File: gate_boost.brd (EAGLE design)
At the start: 74.9 x 45.3 mm, 57 parts, among them IC1 LM324D, IC2 SP34063A_BOOST_REG

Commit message: prior change to charge pump
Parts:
- C1: value (none) -> 1500pf
- R19: value (none) -> 68k
- R20: value (none) -> 180
- R21: value (none) -> 0.22
- R23: value (none) -> 3k3
- R24: value (none) -> 6k2

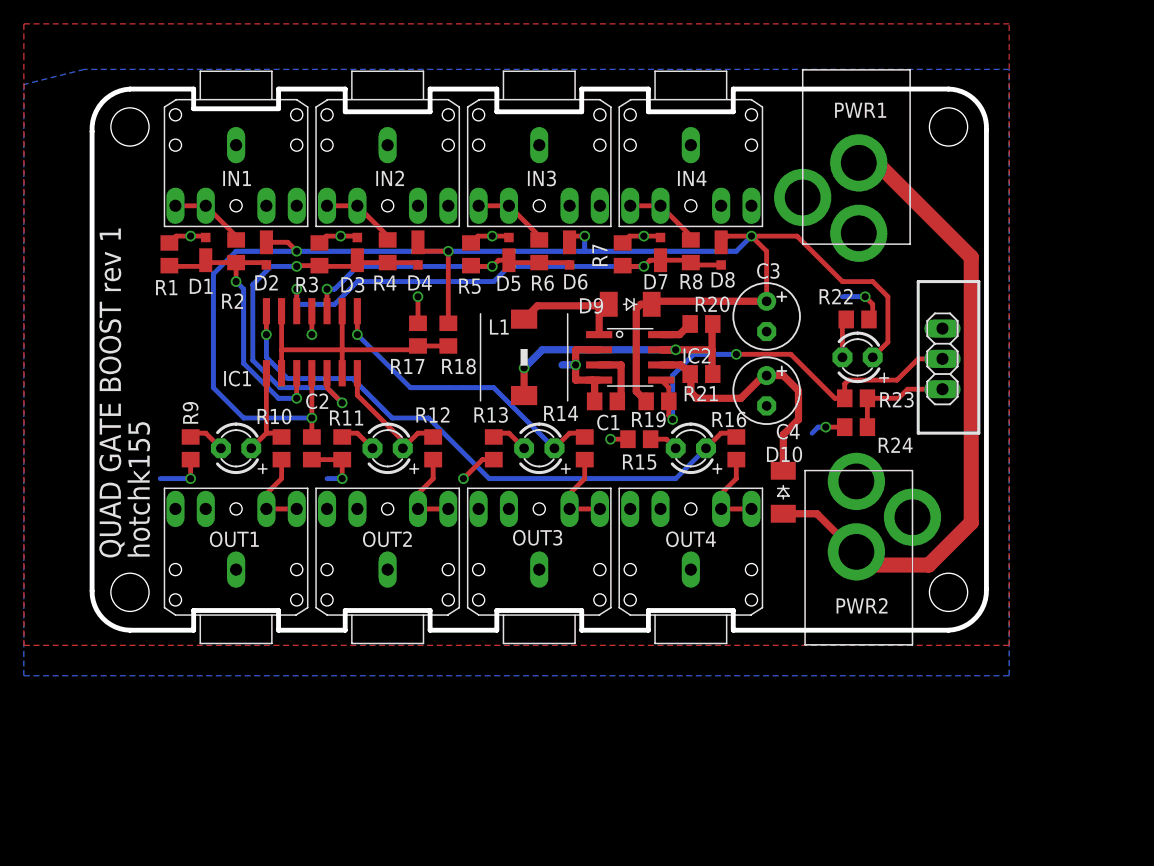
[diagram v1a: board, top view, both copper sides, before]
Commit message: charge pump
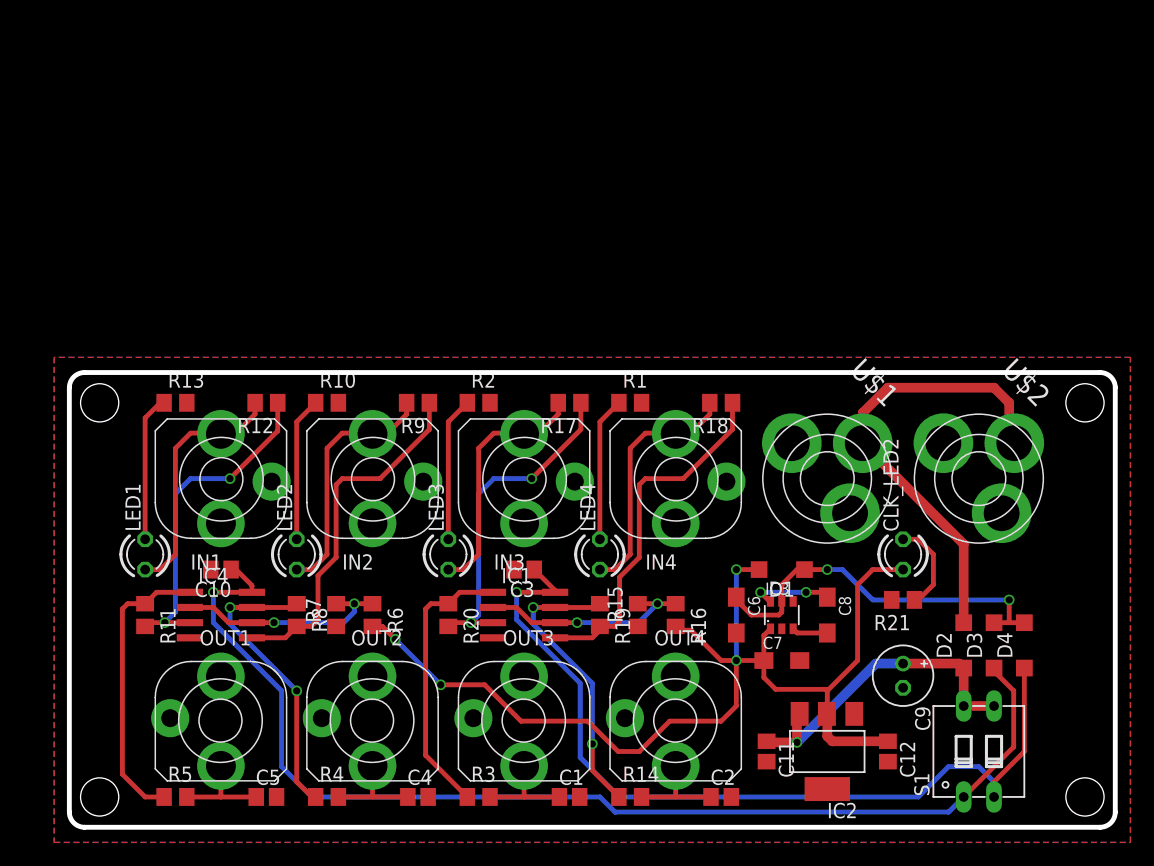
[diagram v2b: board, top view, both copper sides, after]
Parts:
- removed D10, D9: CGRM4001-G, diode:SOD-123_MINI-SMA
- removed D5, D6, D7, D8: PD3S160, diode:POWERDI323
- removed JP1: (no value), pinhead:1X03
- removed L1: (no value), wuerth-elektronik:WE-PD_S/M
- removed LED5: (no value), adafruit:LED3MM
- removed PWR1, PWR2: 2.1MMJACKTHM, adafruit:PJ-102A
- removed R22: (no value), rcl:R0805
- removed R23: 3k3, rcl:R0805
- removed R24: 6k2, rcl:R0805
- added C10, C11, C12, C5: (no value), resistor:C0805
- added C6: (no value), rcl:SMC_A
- added C7, C8: 10u, rcl:SMC_A
- added C9: (no value), rcl:E2-5
- added CLK_LED2: (no value), led:LED3MM
- added IC3: LM27675M5_CHARGEPUMP, jason_eagle6:SOT23-6
- added IC4: LM358D, linear:SO08
- added S1: (no value), switch-dil:DIP02YL
- added U$1, U$2: PWR_SOCKET_2_1MM, jason_eagle6:PWR_SOCKET_2_1MM
- C1: value 1500pf -> (none); device rcl:C0805 -> resistor:C0805
- C2: device rcl:C0805 -> resistor:C0805
- C3, C4: device rcl:E2,5-6 -> resistor:C0805
- D1, D2, D3, D4: value PD3S160 -> MBR0520LT; device diode:POWERDI323 -> diode:SOD123
- IC1: value LM324D -> LM358D; device linear:SO14 -> linear:SO08
- IC2: value SP34063A_BOOST_REG -> REG1117; device jason_eagle6:SOIC8 -> burr-brown:SOT223
- IN1, IN2, IN3, IN4, OUT1, OUT2, OUT3, OUT4: value TRUCONNECTJACK -> VERTICAL_3_5MM_SOCKET; device jason_eagle6:TRUCONNECTJACK -> jason_eagle6:VERTICAL_3_5MM_SOCKET
- LED1, LED2, LED3, LED4: device adafruit:LED3MM -> led:LED3MM
- R1, R10, R13, R2: value (none) -> 1K
- R12, R16, R17, R18, R6, R9: value (none) -> 100k
- R19: value 68k -> (none)
- R20: value 180 -> (none)
- R21: value 0.22 -> 1K
- moved D2 67.1 mm to (72.4, 27.9), turned to 90 degrees
- moved D3 62.7 mm to (74.9, 27.9)
- moved D4 60.6 mm to (77.5, 27.9), turned to 90 degrees
- moved D1 55.1 mm to (57.1, 34.3), turned to 180 degrees
- moved R5 51.8 mm to (6.35, 15.2), turned to 0 degrees
- moved R3 47.4 mm to (31.8, 15.2), turned to 0 degrees
- moved R4 46.0 mm to (19.1, 15.2), turned to 0 degrees
- moved C2 45.0 mm to (52.1, 15.2), turned to 0 degrees
- moved R8 44.9 mm to (16.5, 30.5)
- moved C4 44.9 mm to (26.7, 15.2), turned to 0 degrees
- moved R1 40.6 mm to (44.5, 48.3), turned to 0 degrees
- moved R7 38.6 mm to (19.8, 30.5), turned to 90 degrees
- moved IC2 36.9 mm to (61.0, 19.1), turned to 180 degrees
- moved R6 33.5 mm to (22.9, 30.5)
- moved C1 33.3 mm to (39.4, 15.2), turned to 0 degrees
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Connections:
- removed net N$18: IC1.8, LED3.A, R14.1
- removed net N$22: IC2.8, R20.1
- removed net N$24: C4.+, D10.C, IC2.6, R21.1
- removed net N$25: D10.A, PWR1.RING, PWR2.RING
- removed net N$27: LED1.K, R9.2
- removed net N$30: LED2.K, R11.2
- removed net N$31: LED3.K, R13.2
- removed net N$32: LED4.K, R15.2
- removed net N$34: LED5.K, R22.2
- removed net N$6: D5.C, D6.A, IC1.10, R5.2, R6.2
- removed net V+: C2.2, C3.+, D2.C, D4.C, D6.C, D8.C, D9.C, IC1.4, LED5.A, R18.2, R19.1
- new net +10V: C6.+, D1.C, D3.A, D4.A, IC3.5
- new net +5V: C12.1, C7.+, CLK_LED2.A, D1.A, IC2.2, IC3.1, R16.2, R6.2
- new net IN1: IN1.4, LED1.A, R12.2
- new net IN2: IN2.4, LED2.A, R9.2
- new net IN3: IN3.4, LED3.A, R17.2
- new net IN4: IN4.4, LED4.A, R18.2
- new net N$38: C8.+, IC3.6
- new net N$39: C8.-, IC3.3
- new net VGATE1: C10.1, D3.C, IC4.8, S1.1
- new net VGATE2: C3.1, D4.C, IC1.8, S1.2
- new net VIN: C11.1, C9.+, D2.C, IC2.3, S1.3, S1.4
- net GND: now also C10.2, C11.2, C12.2, C2.2, C3.2, C4.2, C5.2, C6.-, C7.-, C9.-, IC1.4, IC2.1, IC3.2, IC3.4, IC4.4, IN1.2, IN2.2, IN3.2, IN4.2, OUT1.2, OUT2.2, OUT3.2, OUT4.2, R1.2, R10.2, R13.2, R2.2, R21.2, U$1.PIN, U$2.PIN; no longer C2.1, C3.-, C4.-, D1.A, D3.A, D5.A, D7.A, IC1.11, IC2.2, IC2.4, IN1.SLEEVE, IN2.SLEEVE, IN3.SLEEVE, IN4.SLEEVE, OUT1.SLEEVE, OUT2.SLEEVE, OUT3.SLEEVE, OUT4.SLEEVE, PWR1.TIP, PWR2.TIP, R1.1, R11.1, R13.1, R17.1, R22.1, R24.1, R3.1, R5.1, R9.1
- net N$1: now also IC4.2, IC4.6, R6.1, R7.2; no longer IN1.TIP, IN1.TIP_NC, R2.1
- net N$10: now also IC1.7, R14.1, R19.1; no longer IC1.13, IC1.2, IC1.6, IC1.9, R17.2, R18.1
- net N$11: now also IC1.1, R20.1, R3.1; no longer OUT1.TIP, OUT1.TIP_NC, R10.2
- net N$12: now also IC4.7, R4.1, R8.1; no longer OUT2.TIP, OUT2.TIP_NC, R12.2
- net N$13: now also IC1.2, IC1.6, R15.2, R16.1; no longer OUT3.TIP, OUT3.TIP_NC, R14.2
- net N$14: now also LED3.K, R2.1; no longer OUT4.TIP, OUT4.TIP_NC, R16.2
- net N$15: now also LED4.K, R1.1; no longer C1.1, IC2.3
- net N$16: now also IC1.3, R17.1, R20.2; no longer D9.A, IC2.1, L1.2
- net N$17: now also IC1.5, R18.1, R19.2; no longer IC1.7, LED2.A, R12.1
- net N$19: now also C5.1, OUT1.4, R5.2; no longer IC1.14, LED4.A, R16.1
- net N$2: now also LED1.K, R13.1; no longer IN2.TIP, IN2.TIP_NC, R4.1
- net N$20: now also C4.1, OUT2.4, R4.2; no longer IC2.5, JP1.2, R19.2, R23.1
- net N$21: now also D2.A, U$1.BARREL, U$2.BARREL; no longer JP1.1, R23.2, R24.2
- net N$23: now also CLK_LED2.K, R21.1; no longer IC2.7, L1.1, R20.2, R21.2
- net N$3: now also LED2.K, R10.1; no longer IN3.TIP, IN3.TIP_NC, R6.1
- net N$4: now also IC4.3, R11.2, R12.1; no longer IN4.TIP, IN4.TIP_NC, R8.1
- net N$5: now also IC4.5, R9.1; no longer D7.C, D8.A, IC1.12, R7.2
- net N$7: now also C1.1, OUT3.4; no longer D3.C, D4.A, IC1.5, R4.2
- net N$8: now also C2.1, OUT4.4, R14.2; no longer D1.C, D2.A, IC1.3, R1.2, R2.2
- net N$9: now also IC4.1, R11.1, R5.1; no longer IC1.1, LED1.A, R10.1
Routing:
- net V+: track 134.7 -> 0.00 mm, vias 5 -> 0
- net VGATE1: track 0.00 -> 95.6 mm, vias 0 -> 1
- net +5V: track 0.00 -> 91.8 mm, vias 0 -> 4
- net VGATE2: track 0.00 -> 72.7 mm, vias 0 -> 1
- net N$25: track 53.9 -> 0.00 mm
- net GND: track 49.0 -> 0.00 mm, vias 13 -> 0
- net N$19: track 49.2 -> 8.42 mm, vias 1 -> 0
- net +10V: track 0.00 -> 32.0 mm, vias 0 -> 2
- net N$21: track 9.02 -> 38.3 mm
- net VIN: track 0.00 -> 27.6 mm, vias 0 -> 1
- net N$20: track 34.3 -> 8.42 mm, vias 2 -> 0
- net N$18: track 25.6 -> 0.00 mm, vias 1 -> 0
- net N$6: track 25.4 -> 0.00 mm, vias 2 -> 0
- net N$7: track 33.8 -> 8.42 mm, vias 2 -> 0
- net N$24: track 22.2 -> 0.00 mm
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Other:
- board size 74.9 x 45.3 mm -> 87.6 x 38.1 mm
- board text removed: "PWR1"
- board text removed: "PWR2"
- board text removed: "QUAD GATE BOOST rev 1"
- board text removed: "hotchk155"

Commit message: getting there
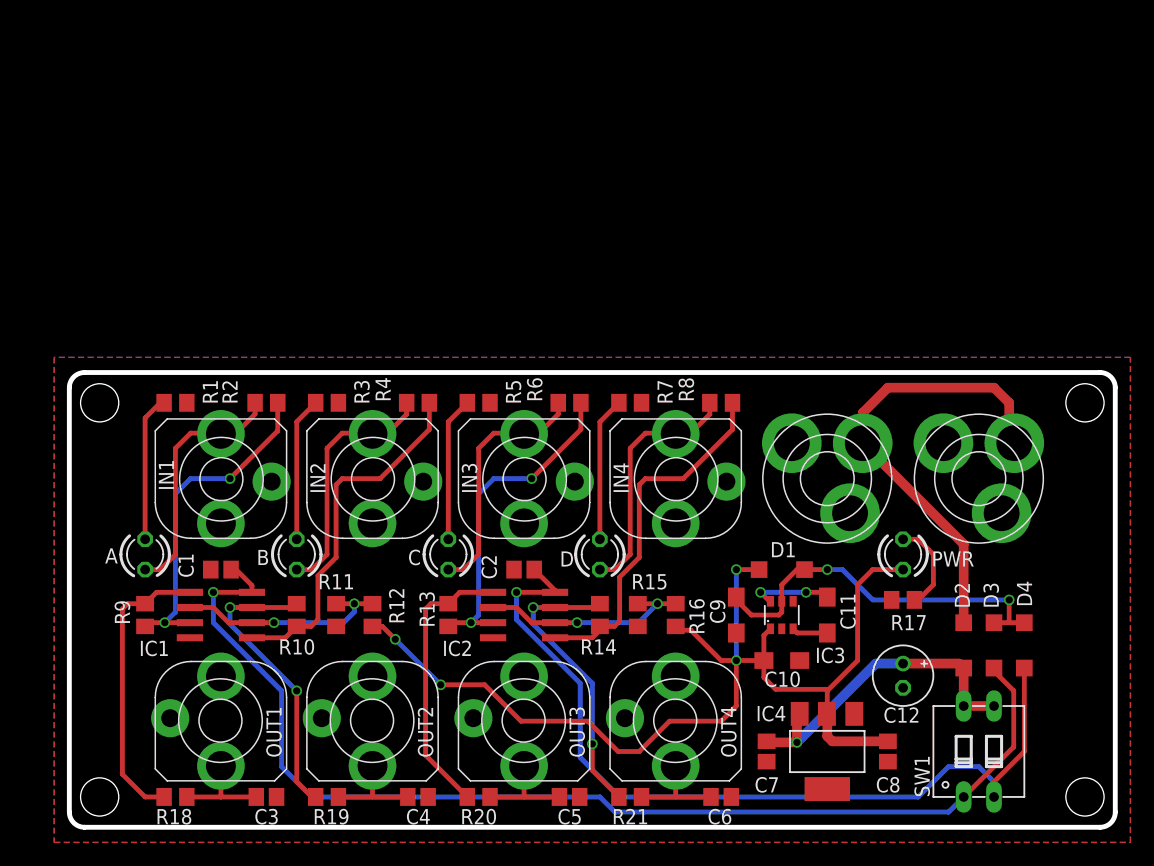
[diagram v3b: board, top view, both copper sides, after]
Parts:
- C10, C11: value (none) -> 10u; device resistor:C0805 -> rcl:SMC_A
- C12: device resistor:C0805 -> rcl:E2-5
- C6: device rcl:SMC_A -> resistor:C0805
- C7, C8: value 10u -> (none); device rcl:SMC_A -> resistor:C0805
- C9: device rcl:E2-5 -> rcl:SMC_A
- IC2: value REG1117 -> LM358D; device burr-brown:SOT223 -> linear:SO08
- IC4: value LM358D -> REG1117; device linear:SO08 -> burr-brown:SOT223
- R10, R13, R21: value 1K -> (none)
- R17: value 100k -> 1K
- R18, R9: value 100k -> (none)
- R2: value 1K -> 100k
- R3, R5, R7: value (none) -> 1K
- R4, R8: value (none) -> 100k
- moved R18 56.4 mm to (6.35, 15.2), turned to 0 degrees
- moved IC4 52.1 mm to (61.0, 19.1), turned to 180 degrees
- moved C10 47.6 mm to (57.1, 26.7), turned to 0 degrees
- moved R5 41.7 mm to (31.8, 48.3)
- moved R8 39.8 mm to (52.1, 48.3), turned to 180 degrees
- moved R1 38.1 mm to (6.35, 48.3)
- moved R3 35.4 mm to (19.1, 48.3)
- moved C1 34.9 mm to (10.2, 34.3), turned to 180 degrees
- moved R4 33.9 mm to (26.7, 48.3), turned to 180 degrees
- moved R17 32.5 mm to (67.3, 31.8)
- moved R7 30.4 mm to (44.5, 48.3), turned to 0 degrees
- moved R13 29.0 mm to (29.2, 30.5), turned to 270 degrees
- moved R9 29.0 mm to (3.81, 30.5), turned to 270 degrees
- moved C3 28.8 mm to (14.0, 15.2), turned to 0 degrees
- moved R21 28.2 mm to (44.5, 15.2), turned to 0 degrees
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- renumbered CLK_LED2 to PWR, LED1 to A, LED2 to B, LED3 to C, LED4 to D, S1 to SW1
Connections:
- net +10V: now also C9.+; no longer C6.+
- net +5V: now also C10.+, C8.1, IC4.2, R12.2; no longer C12.1, C7.+, IC2.2, R6.2
- net GND: now also C10.-, C12.-, C6.2, C7.2, C8.2, IC2.4, IC4.1, R11.1, R17.2, R3.2, R5.2, R7.2; no longer C10.2, C11.2, C12.2, C6.-, C7.-, IC2.1, IC4.4, R10.2, R13.2, R2.2, R21.2, R7.1
- net IN1: now also R2.2; no longer R12.2
- net IN2: now also R4.2; no longer R9.2
- net IN3: now also R6.2; no longer R17.2
- net IN4: now also R8.2; no longer R18.2
- net N$1: now also IC1.2, IC1.6, R11.2, R12.1; no longer IC4.2, IC4.6, R6.1, R7.2
- net N$10: now also IC2.7, R21.1; no longer IC1.7, R19.1
- net N$11: now also IC2.1, R13.1; no longer IC1.1, R3.1
- net N$12: now also IC1.7, R10.1, R19.1; no longer IC4.7, R4.1, R8.1
- net N$13: now also IC2.2, IC2.6; no longer IC1.2, IC1.6
- net N$14: now also R5.1; no longer R2.1
- net N$15: now also R7.1; no longer R1.1
- net N$16: now also IC2.3, R13.2, R6.1; no longer IC1.3, R17.1, R20.2
- net N$17: now also IC2.5, R14.2, R8.1; no longer IC1.5, R18.1, R19.2
- net N$19: now also C3.1, R18.2; no longer C5.1, R5.2
- net N$2: now also R1.1; no longer R13.1
- net N$20: now also R19.2; no longer R4.2
- net N$23: now also R17.1; no longer R21.1
- net N$3: now also R3.1; no longer R10.1
- net N$38: now also C11.+; no longer C8.+
- net N$39: now also C11.-; no longer C8.-
- net N$4: now also IC1.3, R2.1, R9.2; no longer IC4.3, R11.2, R12.1
- net N$5: now also IC1.5, R10.2, R4.1; no longer IC4.5, R8.2, R9.1
- net N$7: now also C5.1, R20.2; no longer C1.1, R3.2
- net N$8: now also C6.1, R21.2; no longer C2.1, R14.2
- net N$9: now also IC1.1, R18.1, R9.1; no longer IC4.1, R11.1, R5.1
- net VGATE1: now also C1.1, IC1.8; no longer C10.1, IC4.8
- net VGATE2: now also C2.1, IC2.8; no longer C3.1, IC1.8
- net VIN: now also C12.+, C7.1, IC4.3; no longer C11.1, C9.+, IC2.3
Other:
- board text added: "CV.OCD Gate Boost v1"
- board text added: "six4pix.com/cvocd"

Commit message: component values
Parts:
- R13, R14: value (none) -> 2m2
- R15: value (none) -> 47k
- R16: value 100k -> 47k
- R20, R21: value (none) -> 1k

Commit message: aye
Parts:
- R10, R9: value (none) -> 2m2
- R11: value (none) -> 47k
- R12: value 100k -> 47k
- R18, R19: value (none) -> 1k
